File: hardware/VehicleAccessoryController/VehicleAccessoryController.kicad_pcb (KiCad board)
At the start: 4 copper layers, 61.4 x 75.2 mm, 81 parts, among them J501 Input, J502 Front Conn, J503 Rear Conn, J504 Left Conn, J505 Right Conn, J506 USB_B_Mini, P601 TC2030-MCP, Q201 BSS138, Q202 BSS138, Q203 BSS138, Q204 BSS138, SW301 ON/OFF, U101 RECOM_REMX0-W, U102 ATMEGA328P-M(32QFN_MLF), U103 TPS3710, U104 SI8710CC-B-IS, U105 CP2102N-A02-GQFN24, U106 Si8631EC-B-IS1, U107 NCV551SN50T1G, Y901 16MHz

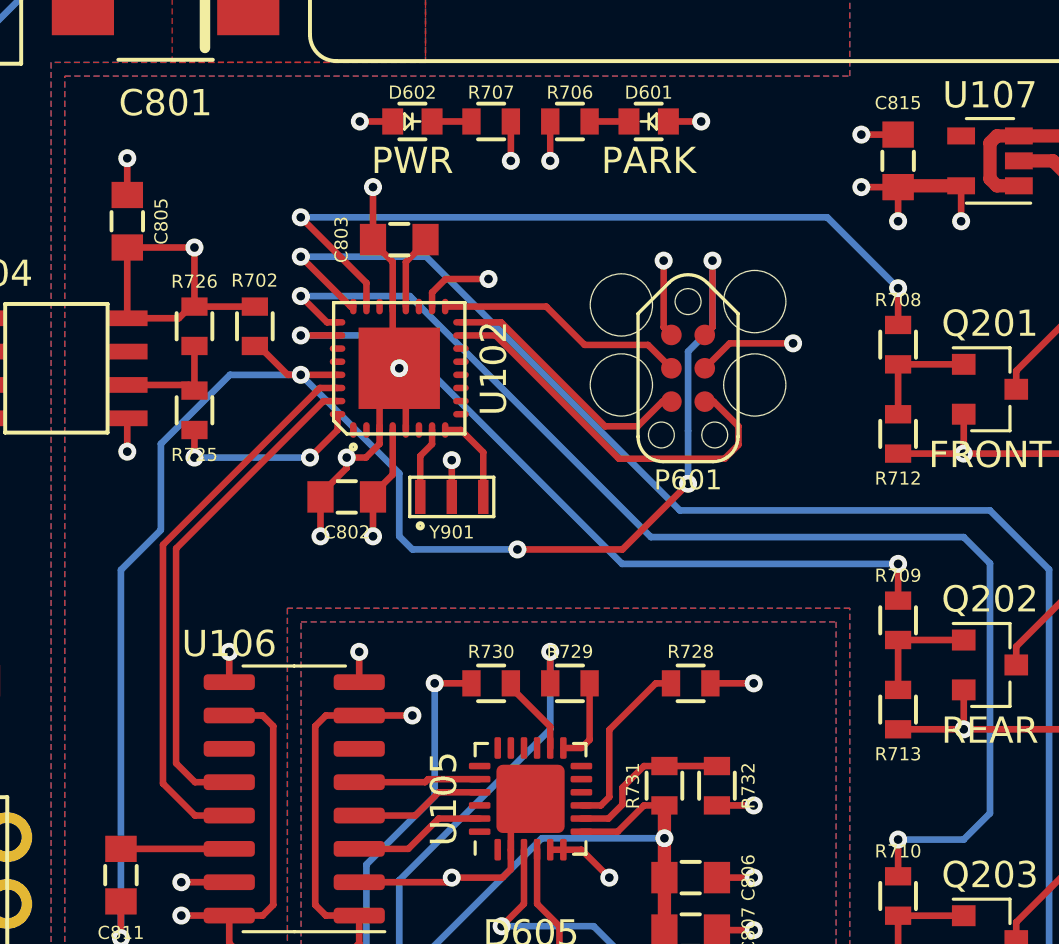
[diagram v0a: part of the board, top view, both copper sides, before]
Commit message: schematic/layout updates
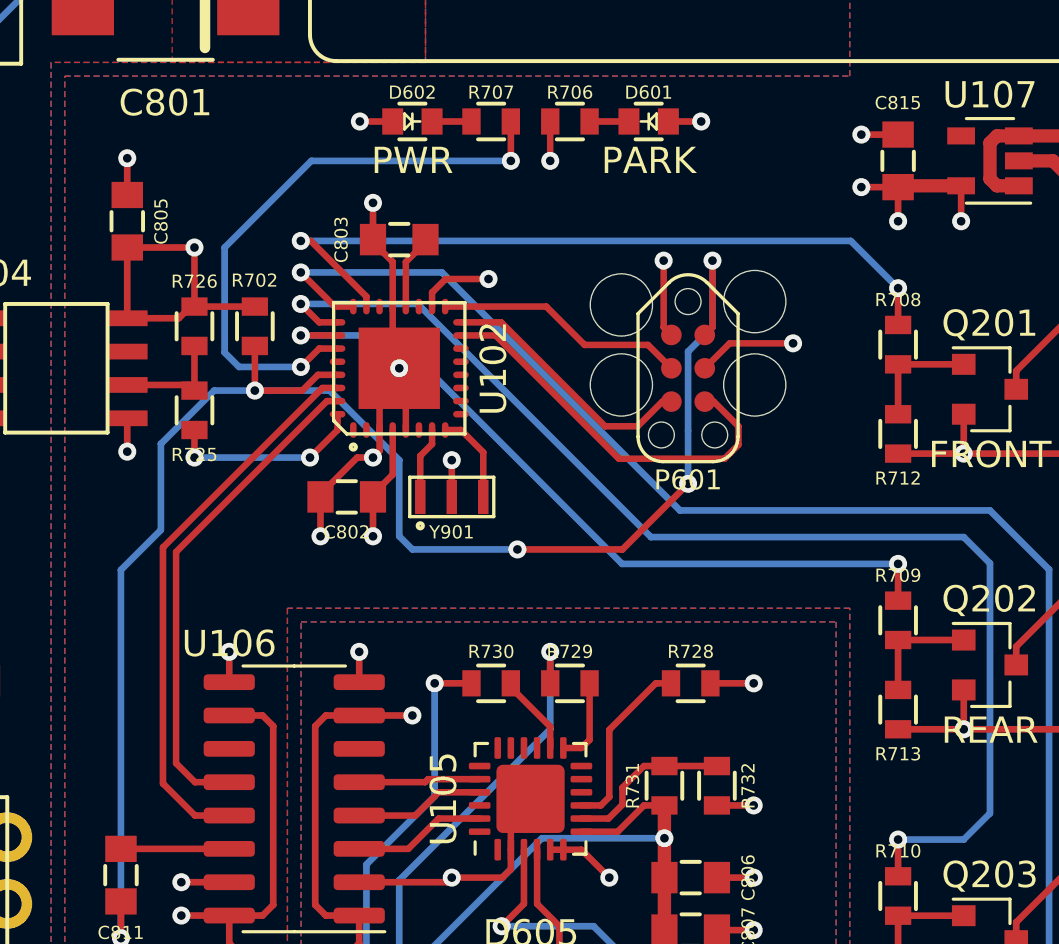
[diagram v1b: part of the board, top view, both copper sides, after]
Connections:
- U102 pad 19: /PARK_STATUS -> (no net)
- U102 pad 22: /POWER_STATUS -> /PARK_STATUS
- U102 pad 27: Net-(U102-Pad27) -> /POWER_STATUS
- U102 pad 28: Net-(U102-Pad28) -> (no net)
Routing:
- net /POWER_STATUS: track 1.50 -> 22.6 mm, vias 1 -> 2
- net /328P_RST: track 62.8 -> 64.1 mm
- net /PARK_FRONT: track 29.7 -> 28.7 mm
- net GND: track 76.4 -> 75.8 mm
